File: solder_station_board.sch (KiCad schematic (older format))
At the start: 43 parts, among them J7 ROTARY, J8 SERIAL, P1 ISP, U4 MAX31855KASA

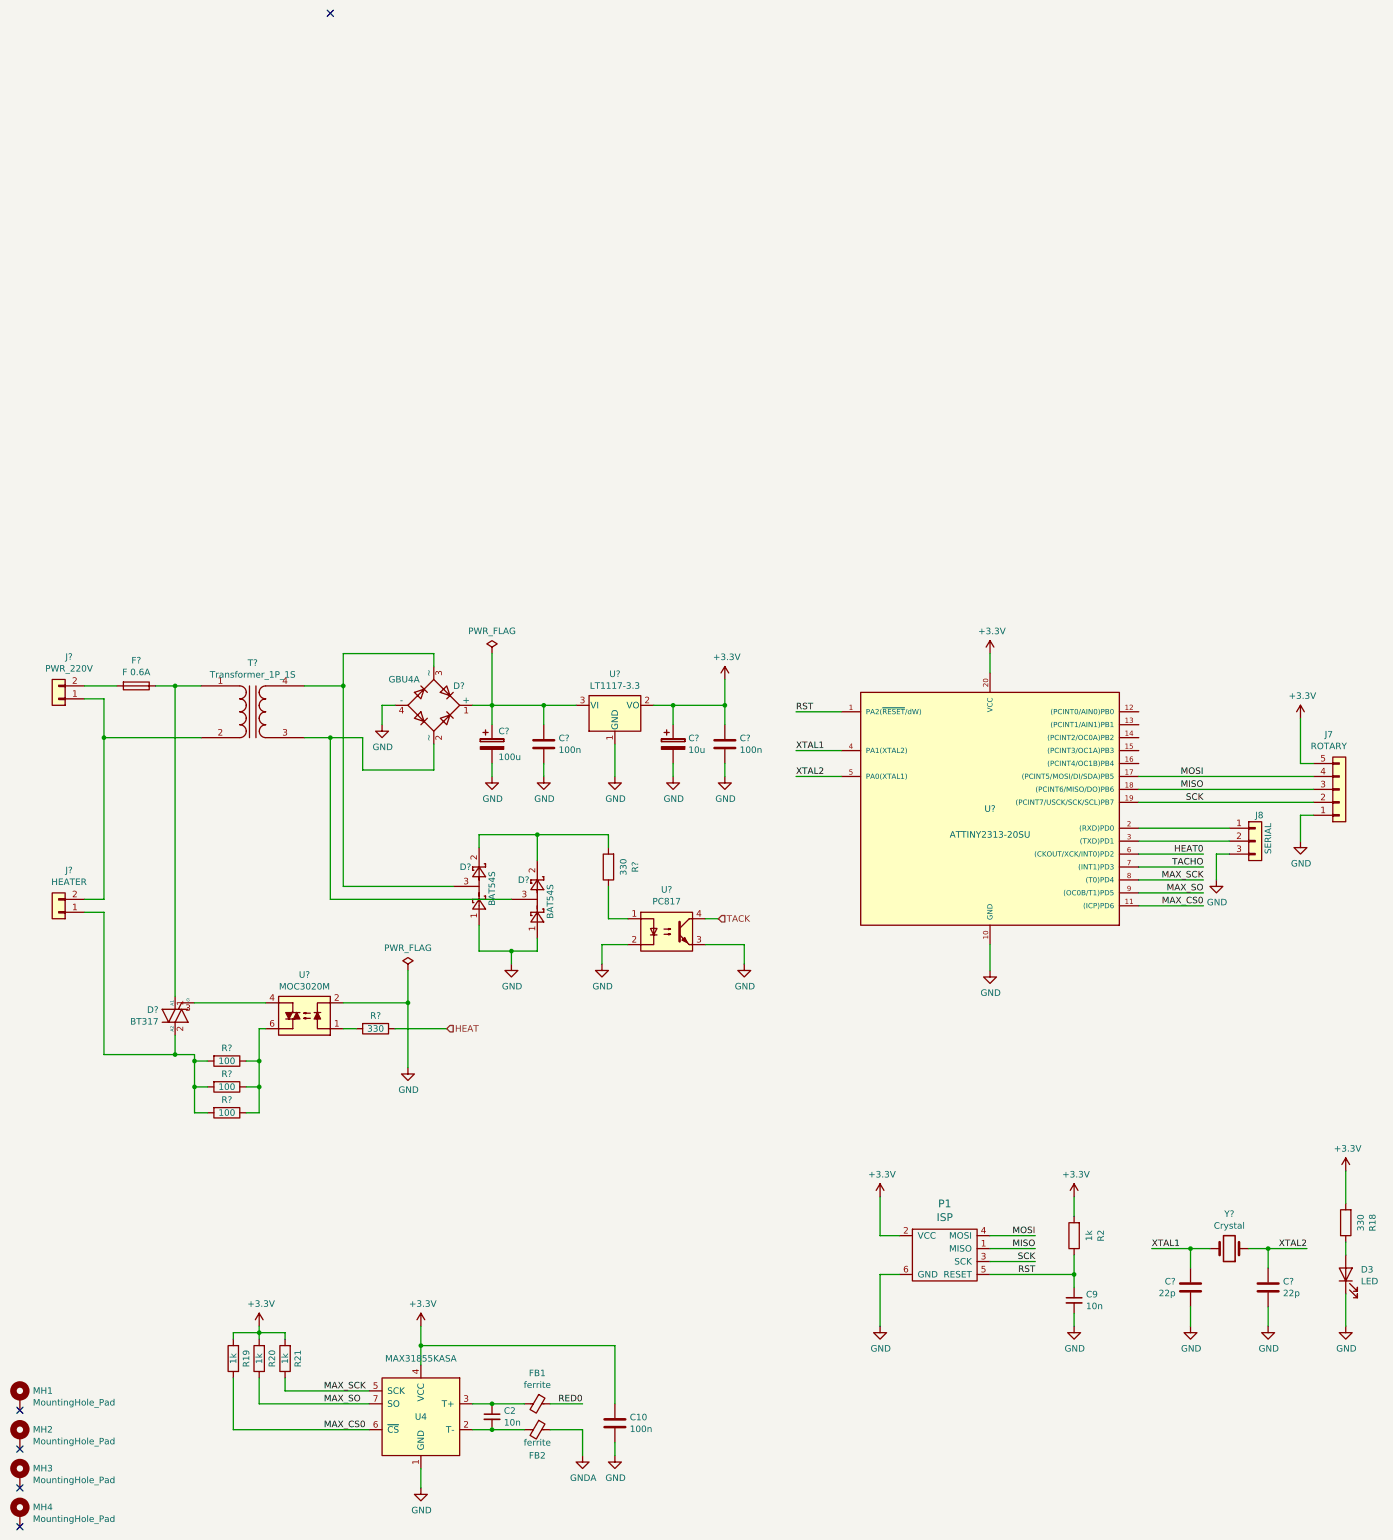
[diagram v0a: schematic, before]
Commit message: place
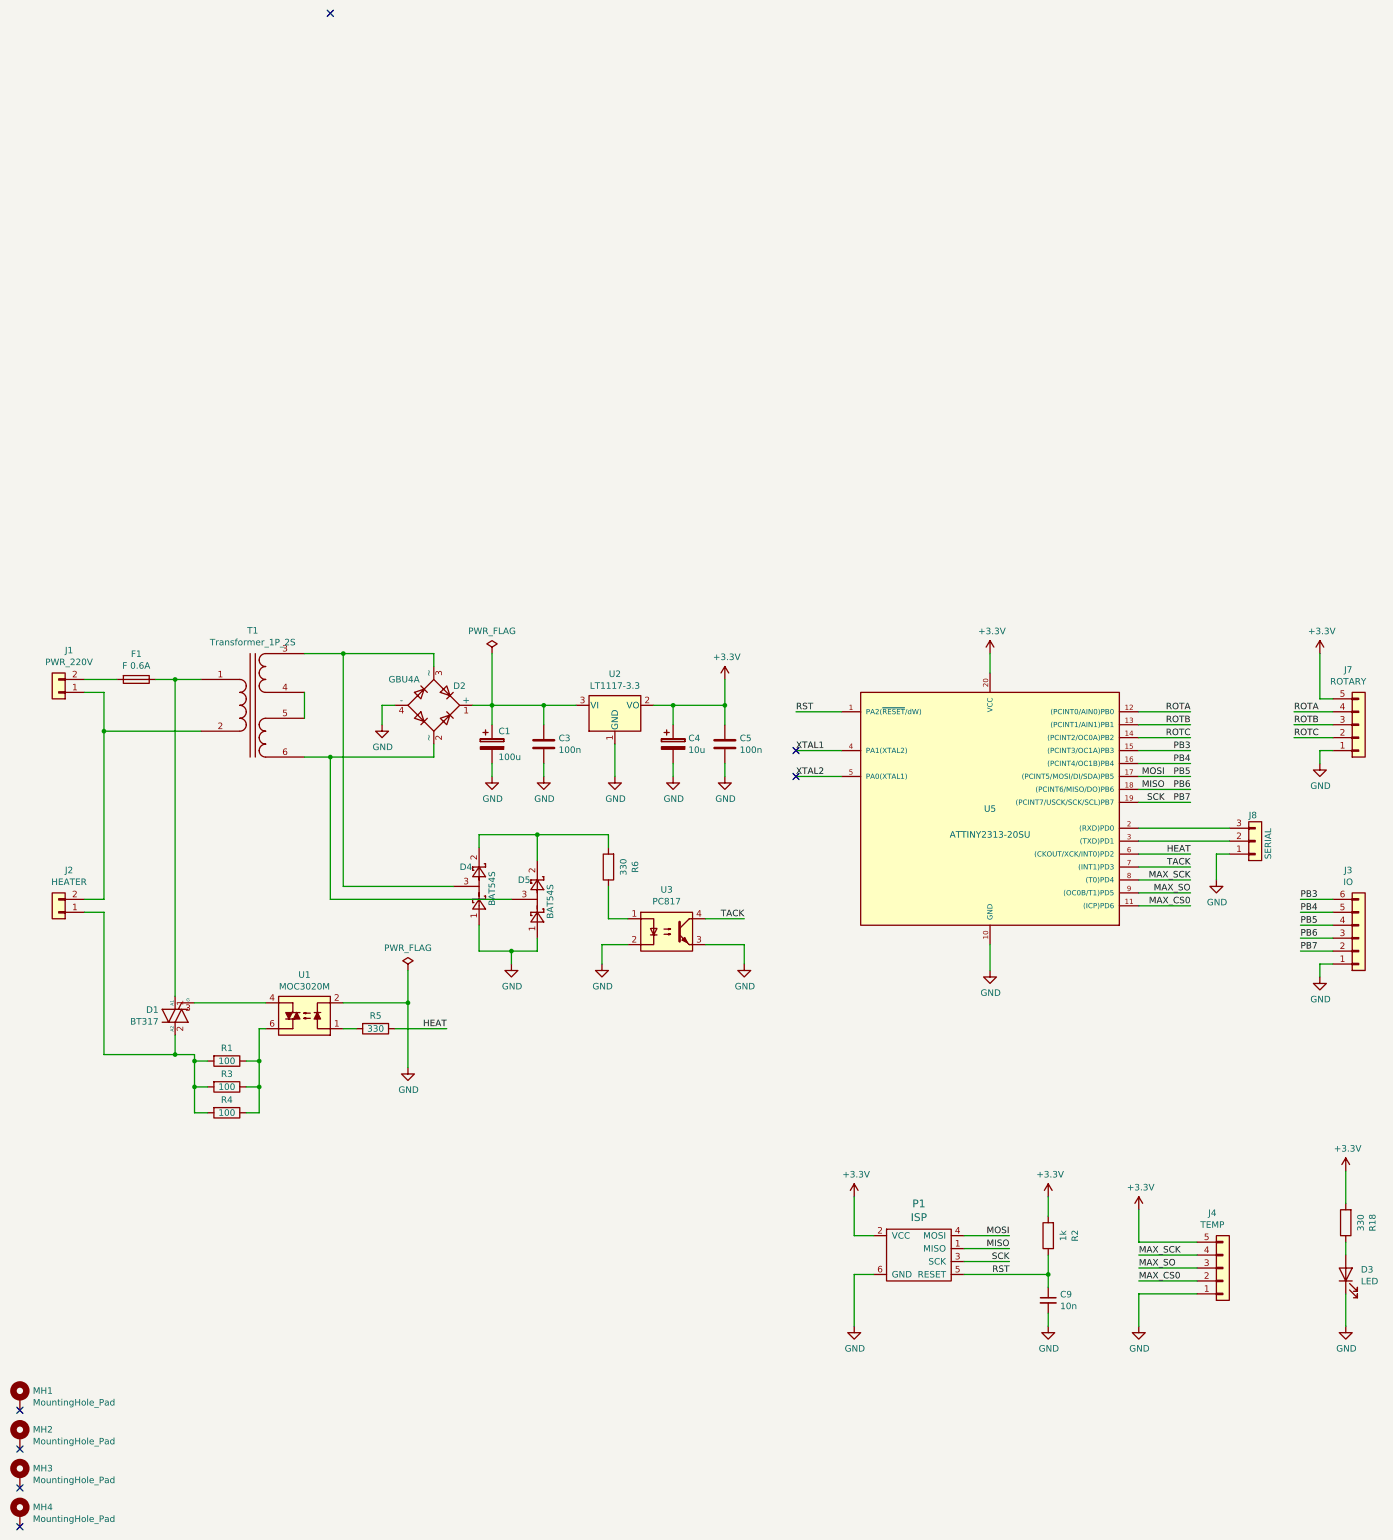
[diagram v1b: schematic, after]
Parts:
- removed C10: 100n, Capacitor_SMD:C_0805_2012Metric_Pad1.15x1.40mm_HandSolder, symbol solder_station_board-rescue:C-Device
- removed C2: 10n, Capacitor_SMD:C_0603_1608Metric_Pad1.05x0.95mm_HandSolder, symbol Device:C_Small
- removed C? (x2): 22p, symbol Device:C
- removed FB1, FB2: ferrite, Inductor_SMD:L_0805_2012Metric_Pad1.15x1.40mm_HandSolder, symbol Device:Ferrite_Bead_Small
- removed R19, R20, R21: 1k, Resistor_SMD:R_0603_1608Metric_Pad1.05x0.95mm_HandSolder, symbol solder_station_board-rescue:R-Device
- removed T?: Transformer_1P_1S, symbol Device:Transformer_1P_1S
- removed U4: MAX31855KASA, Package_SO:SOIC-8_3.9x4.9mm_P1.27mm, symbol solder_station_board-rescue:MAX31855KASA-Sensor_Temperature
- removed Y?: Crystal, symbol Device:Crystal
- added J3: IO, Connector_JST:JST_XH_B6B-XH-A_1x06_P2.50mm_Vertical, symbol Connector_Generic:Conn_01x06
- added J4: TEMP, Connector_JST:JST_XH_B5B-XH-A_1x05_P2.50mm_Vertical, symbol solder_station_board-rescue:Conn_01x05-Connector_Generic
- added T1: Transformer_1P_2S, custom:TRAFO_1P_2S, symbol Device:Transformer_1P_2S
- D1: renamed from D?; footprint (none) -> Package_TO_SOT_THT:TO-126-3_Vertical
- D3: footprint LED_SMD:LED_0603_1608Metric_Castellated -> LED_THT:LED_D3.0mm
- F1: renamed from F?; footprint (none) -> custom:Fuseholder_Cylinder-5x20mmP1.5_Schurter_0031_8201_Horizontal_Open
- R1, R3, R4: renamed from R?; footprint (none) -> Resistor_SMD:R_1206_3216Metric
- R5: renamed from R?; footprint (none) -> Resistor_SMD:R_0603_1608Metric_Pad1.05x0.95mm_HandSolder
- U1: renamed from U?; footprint (none) -> Package_DIP:DIP-6_W7.62mm_LongPads
- U5: renamed from U?; footprint Housings_SOIC:SOIC-20W_7.5x12.8mm_Pitch1.27mm -> Package_SO:SOIC-20W_7.5x12.8mm_P1.27mm
- gave numbers to parts that had none: 12
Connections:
- net HEAT0 is gone; now on net HEAT: U5.6 ((CKOUT/XCK/INT0)PD2)
- net TACHO is gone; now on net TACK: U5.7 ((INT1)PD3)
- net +3V3: now also J4.5 (Pin_5)
- net GND: now also J8.1 (Pin_1), J3.1 (Pin_1), J4.1 (Pin_1); no longer J8.3 (Pin_3)
- net MAX_CS0: now also J4.2 (Pin_2)
- net MAX_SCK: now also J4.4 (Pin_4)
- net MAX_SO: now also J4.3 (Pin_3)
- net MISO: now also J3.3 (Pin_3); no longer J7.3 (Pin_3)
- net MOSI: now also J3.4 (Pin_4); no longer J7.4 (Pin_4)
- net at U5.2 ((RXD)PD0): now also J8.3 (Pin_3); no longer J8.1 (Pin_1)
- net ROTA: now reaches U5.12 ((PCINT0/AIN0)PB0)
- net ROTA: now also J7.4 (Pin_4)
- net ROTB: now reaches U5.13 ((PCINT1/AIN1)PB1)
- net ROTB: now also J7.3 (Pin_3)
- net ROTC: now reaches U5.14 ((PCINT2/OC0A)PB2)
- net ROTC: now also J7.2 (Pin_2)
- net PB3: now reaches U5.15 ((PCINT3/OC1A)PB3)
- net PB3: now also J3.6 (Pin_6)
- net PB4: now reaches U5.16 ((PCINT4/OC1B)PB4)
- net PB4: now also J3.5 (Pin_5)
- net at J1.1 (Pin_1), J2.2 (Pin_2): now also T1.2 (AB)
- net at D2.2 (~~), D5.3: now also T1.6 (SD)
- net at D2.3 (~~), D4.3: now also T1.3 (SA)
- net at D1.1 (A1), F1.1: now also T1.1 (AA)
- net SCK renamed PB7
- net PB7: now also J3.2 (Pin_2); no longer J7.2 (Pin_2)
- new net: T1.4 (SB), T1.5 (SC)
- no-connect marks 5 -> 7
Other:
- moved on the sheet: C9, F1, J1, J7, P1, R2
